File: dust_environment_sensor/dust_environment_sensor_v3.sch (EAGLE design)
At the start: 38 parts, among them IC2 ATMEGA644A, J1 3.6V Lithium C cell, J3 XBEE_1-10SMT, J4 XBEE_11-20SMT, U1 TSL2560T, U2 LIS3DH, U4 HTU21D, U5 AMN41121, U7 MCP1700-3.3V, X2 32.768KHz

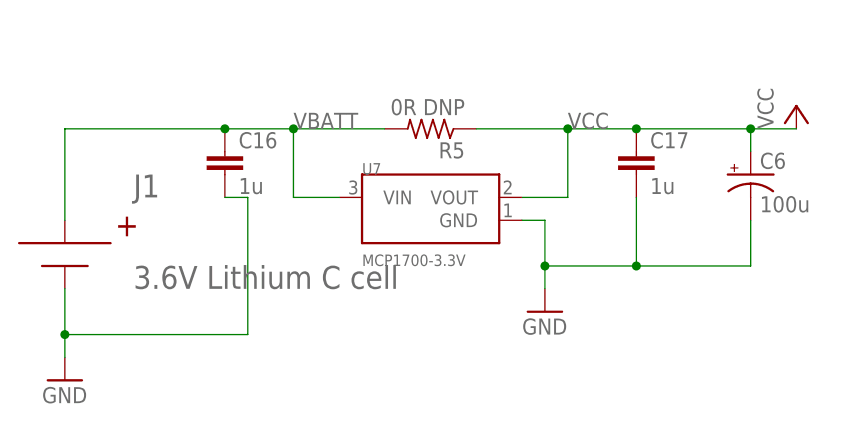
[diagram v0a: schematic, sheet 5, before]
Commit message: Updated board design and shipping
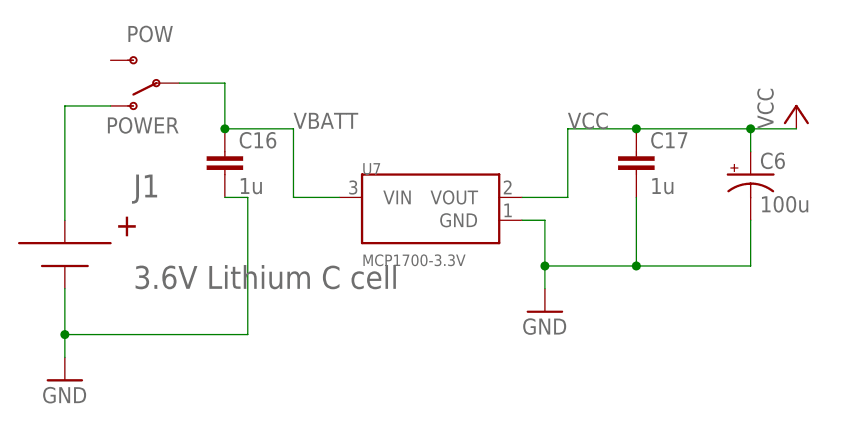
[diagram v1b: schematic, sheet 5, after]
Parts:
- removed R5: 0R DNP, resistor:R-US_R0603
- added POW: POWER, Cool_Electricity:SWITCH-SPDTSMD3
- EXP: value M05X2SHD -> M05X2SHD_SMD; device SparkFun-Connectors:M05X2SHD -> SparkFun-Connectors:M05X2SHD_SMD
- JP9: device SparkFun-Connectors:M05X2SHD -> SparkFun-Connectors:M05X2SHD_SMD
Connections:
- new net N$1: J1.POS, POW.O
- net VBATT: now also POW.P; no longer J1.POS, R5.2
- net VCC: no longer R5.1
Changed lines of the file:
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@@
 <part name="JP8" library="custom" deviceset="FTDI_CABLE" device="SIP"/>
 <part name="GND21" library="SparkFun" deviceset="GND" device=""/>
-<part name="JP9" library="SparkFun-Connectors" deviceset="M05X2" device="SHD" value="JTAG"/>
+<part name="JP9" library="SparkFun-Connectors" deviceset="M05X2" device="SHD_SMD" value="JTAG"/>
 <part name="GND24" library="SparkFun" deviceset="GND" device=""/>
 <part name="P+3" library="supply1" deviceset="VCC" device=""/>
@@
 <part name="R4" library="resistor" deviceset="R-US_" device="R0603" value="10k"/>
 <part name="P+9" library="supply1" deviceset="VCC" device=""/>
-<part name="R5" library="resistor" deviceset="R-US_" device="R0603" value="0R DNP"/>
 <part name="P+10" library="supply1" deviceset="VCC" device=""/>
 <part name="U5" library="Cool_Electricity" deviceset="AMN41121" device=""/>
@@
 <part name="P+1" library="supply1" deviceset="VCC" device=""/>
 <part name="C3" library="rcl" deviceset="C-EU" device="C0603" value="100n"/>
-<part name="EXP" library="SparkFun-Connectors" deviceset="M05X2" device="SHD"/>
+<part name="EXP" library="SparkFun-Connectors" deviceset="M05X2" device="SHD_SMD" value="M05X2SHD_SMD"/>
 <part name="GND10" library="SparkFun" deviceset="GND" device=""/>
 <part name="U4" library="Cool_Electricity" deviceset="HTU21D" device=""/>
@@
 <part name="JP2" library="SparkFun-Connectors" deviceset="M02" device="PTH"/>
 <part name="GND3" library="SparkFun" deviceset="GND" device=""/>
+<part name="POW" library="Cool_Electricity" deviceset="SWITCH-SPDT" device="SMD3" value="POWER"/>
 </parts>
 <sheets>
@@
 <instance part="J1" gate="G$1" x="22.86" y="33.02"/>
 <instance part="GND7" gate="1" x="22.86" y="20.32"/>
-<instance part="R5" gate="G$1" x="63.5" y="48.26" rot="R180"/>
 <instance part="P+10" gate="VCC" x="104.14" y="50.8"/>
 <instance part="U7" gate="G$1" x="63.5" y="38.1"/>
@@
 <instance part="C17" gate="G$1" x="86.36" y="45.72"/>
 <instance part="C6" gate="G$1" x="99.06" y="43.18"/>
+<instance part="POW" gate="1" x="33.02" y="53.34" rot="R180"/>
 </instances>
 <busses>
@@
 <net name="VCC" class="0">
 <segment>
-<pinref part="R5" gate="G$1" pin="1"/>
-<wire x1="68.58" y1="48.26" x2="78.74" y2="48.26" width="0.1524" layer="91"/>
 <label x="78.74" y="48.26" size="1.778" layer="95"/>
 <pinref part="P+10" gate="VCC" pin="VCC"/>
@@
 <wire x1="73.66" y1="40.64" x2="78.74" y2="40.64" width="0.1524" layer="91"/>
 <wire x1="78.74" y1="40.64" x2="78.74" y2="48.26" width="0.1524" layer="91"/>
-<junction x="78.74" y="48.26"/>
 <pinref part="C17" gate="G$1" pin="1"/>
 <junction x="86.36" y="48.26"/>
@@
 <net name="VBATT" class="0">
 <segment>
-<pinref part="J1" gate="G$1" pin="POS"/>
-<wire x1="22.86" y1="38.1" x2="22.86" y2="48.26" width="0.1524" layer="91"/>
-<wire x1="22.86" y1="48.26" x2="40.64" y2="48.26" width="0.1524" layer="91"/>
 <label x="48.26" y="48.26" size="1.778" layer="95"/>
-<pinref part="R5" gate="G$1" pin="2"/>
 <pinref part="U7" gate="G$1" pin="VIN"/>
 <wire x1="40.64" y1="48.26" x2="48.26" y2="48.26" width="0.1524" layer="91"/>
-<wire x1="48.26" y1="48.26" x2="58.42" y2="48.26" width="0.1524" layer="91"/>
 <wire x1="53.34" y1="40.64" x2="48.26" y2="40.64" width="0.1524" layer="91"/>
 <wire x1="48.26" y1="40.64" x2="48.26" y2="48.26" width="0.1524" layer="91"/>
-<junction x="48.26" y="48.26"/>
 <pinref part="C16" gate="G$1" pin="1"/>
+<pinref part="POW" gate="1" pin="P"/>
+<wire x1="35.56" y1="53.34" x2="40.64" y2="53.34" width="0.1524" layer="91"/>
+<wire x1="40.64" y1="53.34" x2="40.64" y2="48.26" width="0.1524" layer="91"/>
 <junction x="40.64" y="48.26"/>
 </segment>
 </net>
+<net name="N$1" class="0">
+<segment>
+<pinref part="J1" gate="G$1" pin="POS"/>
+<wire x1="22.86" y1="38.1" x2="22.86" y2="50.8" width="0.1524" layer="91"/>
+<pinref part="POW" gate="1" pin="O"/>
+<wire x1="22.86" y1="50.8" x2="27.94" y2="50.8" width="0.1524" layer="91"/>
+</segment>
+</net>
